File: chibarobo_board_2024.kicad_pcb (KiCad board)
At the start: 2 copper layers, 100 x 70 mm, 144 parts, among them IC1 ESP32-S2-DevKitM-1, IC2 NCP3020ADR2G, IC3 TC74HC00AF_F_, IC4 L78M05CDT, IC5 TC7W14FK, J1 Conn_01x14_Socket, J10 Conn_01x03_Socket, J11 Conn_01x02_Socket, J12 Conn_01x03_Socket, J13 Conn_01x03_Socket, J14 Conn_01x03_Socket, J15 Conn_01x02_Socket, J16 Conn_01x02_Socket, J2 Conn_01x03_Socket, J3 Conn_01x03_Socket, J4 Conn_01x03_Socket, J5 Conn_01x03_Socket, J6 Conn_01x03_Socket, J7 Conn_01x02_Socket, J8 Conn_01x03_Socket, J9 Conn_01x02_Socket, K1 V23134J, Q1 IRFIZ24NPbF, Q10 2SC2712-GR_TE85L,F, Q11 2SC2712-GR_TE85L,F, Q12 2SC2712-GR_TE85L,F, Q13 2SC2712-GR_TE85L,F, Q14 IRFL014TRPBF, Q15 NTA7002NT1G, Q2 IRFR014TRPBF-BE3, Q3 2SA1162-GR_F_, Q4 2SA1162-GR_F_, Q5 2SA1162-GR_F_, Q6 2SA1162-GR_F_, Q7 2SA1162-GR_F_, Q8 2SA1162-GR_F_, Q9 2SC2712-GR_TE85L,F, U1 TLP291, U2 TLP291, U3 TLP291, U4 TLP291, U5 TLP291, U6 74LVC1G123, U7 TLP291, U8 TSM3446CX6

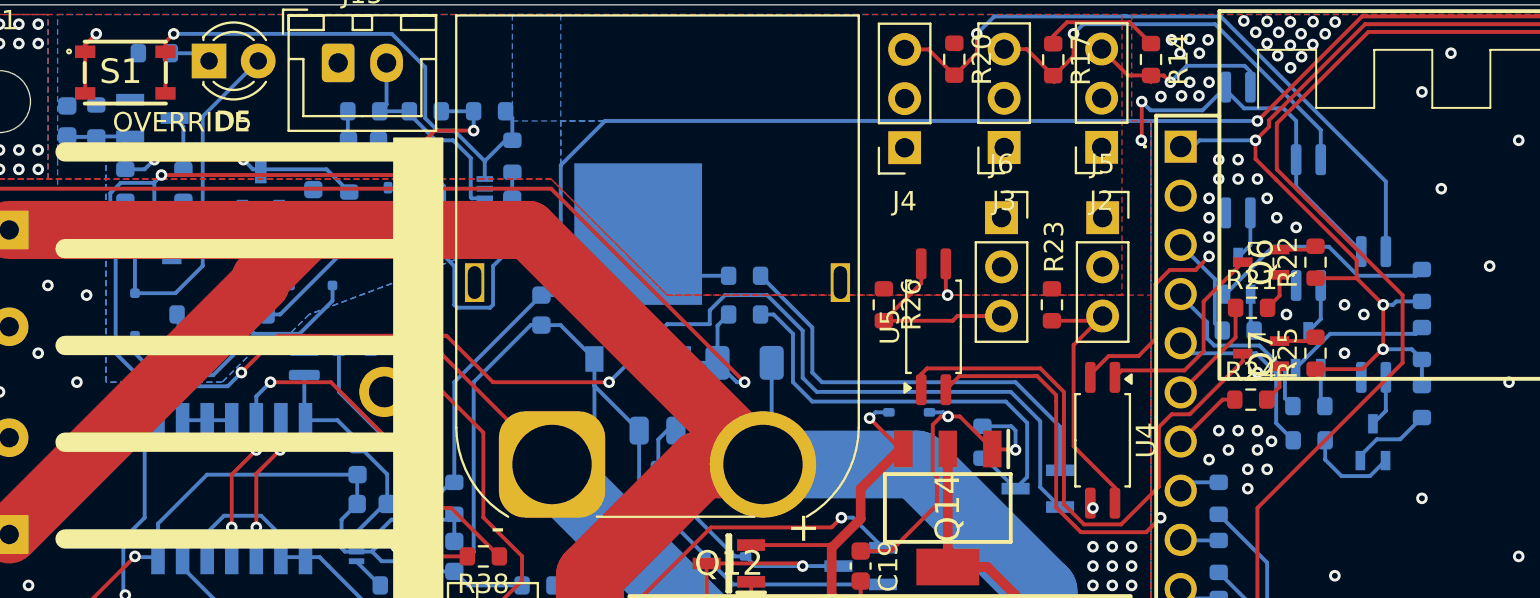
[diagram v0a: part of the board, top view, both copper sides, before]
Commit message: Rev1
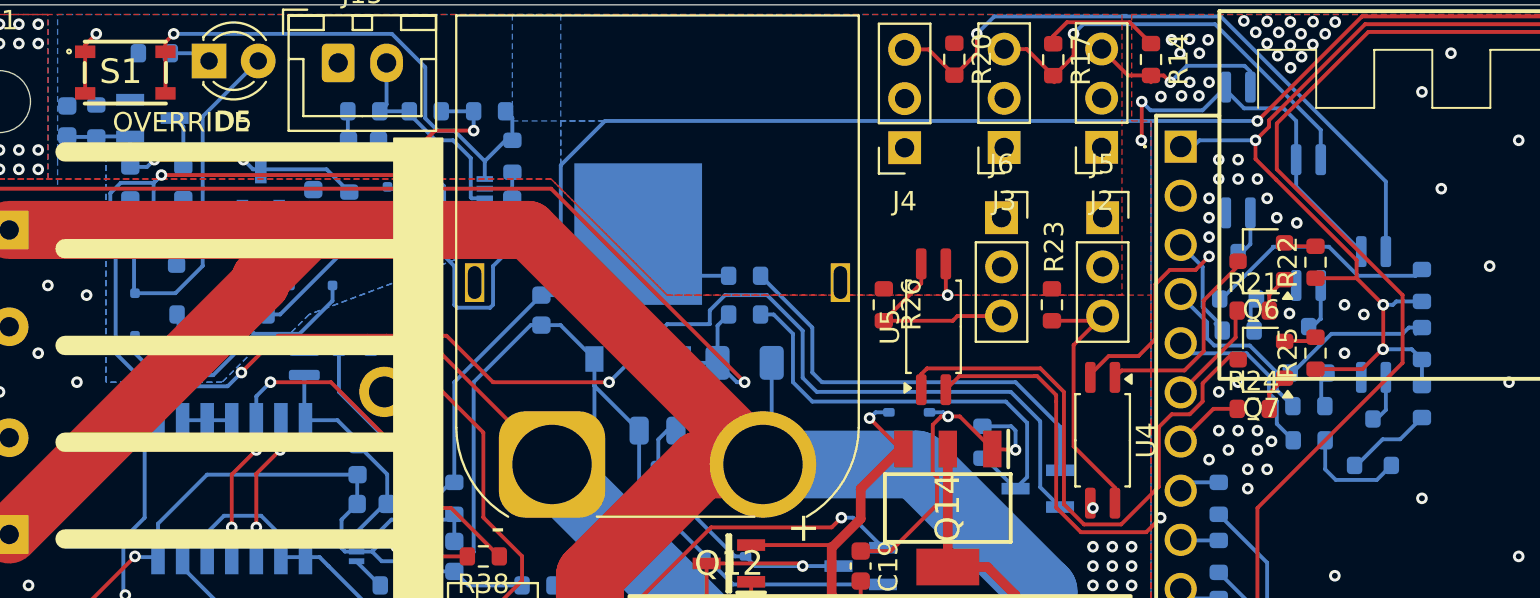
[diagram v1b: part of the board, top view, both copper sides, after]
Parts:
- D4: footprint Diode_SMD:D_SOD-323 -> Diode_SMD:D_SOD-323F
- Q3, Q4, Q5, Q6, Q7, Q8: footprint SamacSys_Parts:SSM3K7002CFULF -> Package_TO_SOT_SMD:SC-59
- moved R24 0.49 mm to (169.8, 70.9)
- moved Q7 0.32 mm to (170.2, 68.3), turned to 180 degrees
- moved R43 0.29 mm to (111.8, 59.2)
- moved R21 0.17 mm to (169.8, 65.8)
- moved R47 0.14 mm to (114.5, 59.2)
- turned Q6 to 180 degrees
- turned Q4 to 90 degrees
- turned Q3 to 90 degrees
- turned Q5 to 90 degrees
- turned Q8 to 180 degrees
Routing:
- net Net-(Q5-Pad1): track 4.80 -> 5.46 mm
- net Net-(Q10-COLLECTOR): track 17.6 -> 17.0 mm
- net Net-(Q8-Pad1): track 1.95 -> 2.46 mm
- net /Servo/Servo1: track 5.31 -> 5.82 mm
- net GND: vias 86 -> 87
